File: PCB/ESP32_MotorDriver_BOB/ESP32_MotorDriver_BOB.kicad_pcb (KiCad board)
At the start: 4 copper layers, 30.5 x 58.4 mm, 39 parts, among them J1 USB_C_Receptacle_USB2.0, J2 Conn_01x06, J3 Conn_01x06, J5 Conn_01x18, J6 Conn_01x07, Q1 SSM3J338R_LF, SW1 RESET, SW2 BOOT, U1 ESP32-S2-SOLO-N4, U2 D3V3XA4B10LP, U4 TB6612FNG, U5 AP63203WU

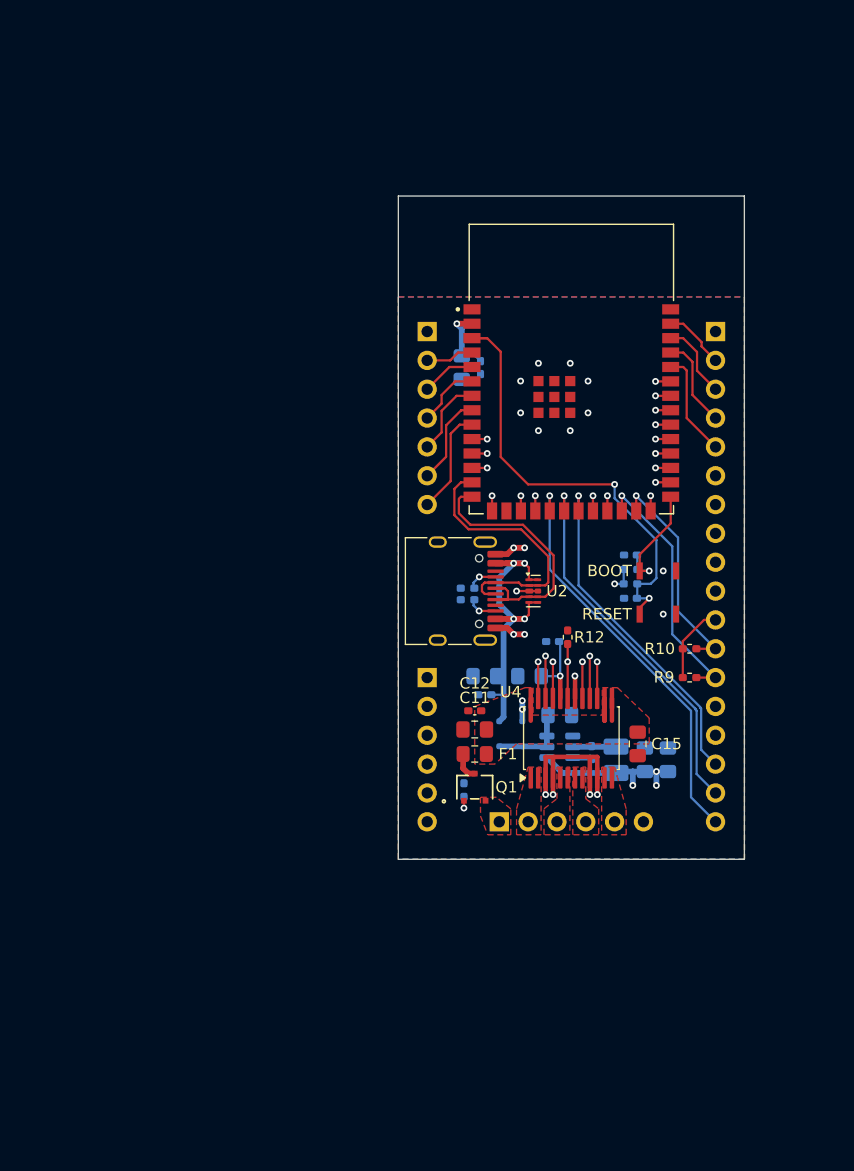
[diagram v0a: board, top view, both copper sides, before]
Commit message: actual _v01
Issue with files being copied - these should be good
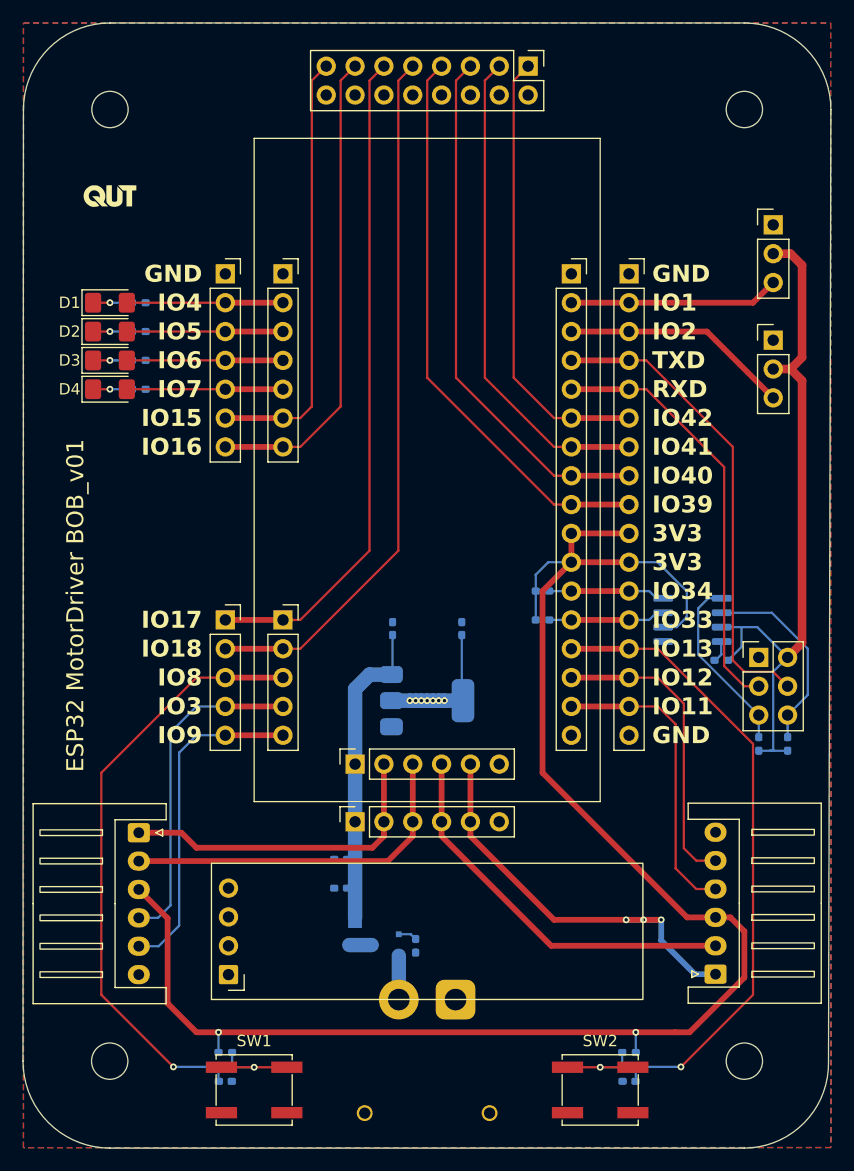
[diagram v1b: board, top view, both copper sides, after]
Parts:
- removed C1, C3, C5, C7: 10uF, Capacitor_SMD:C_0805_2012Metric_Pad1.18x1.45mm_HandSolder
- removed C10, C9: 22uF, Capacitor_SMD:C_0805_2012Metric_Pad1.18x1.45mm_HandSolder
- removed C2, C4, C6, C8: 100nF, Capacitor_SMD:C_0402_1005Metric_Pad0.74x0.62mm_HandSolder
- removed L1: 4.7uH, Inductor_SMD:L_1008_2520Metric_Pad1.43x2.20mm_HandSolder
- removed U5: AP63203WU, Package_TO_SOT_SMD:TSOT-23-6
- added C16: 100nF, Capacitor_SMD:C_0402_1005Metric_Pad0.74x0.62mm_HandSolder, B.Cu at (132.1, 113.5)
- added D3: BLUE, LED_SMD:LED_1206_3216Metric_Pad1.42x1.75mm_HandSolder, F.Cu at (86.4, 50.0)
- added D4: YELLOW, LED_SMD:LED_1206_3216Metric_Pad1.42x1.75mm_HandSolder, F.Cu at (86.4, 52.6)
- added H1: MountingHole, MountingHole:MountingHole_3.2mm_M3, F.Cu at (86.4, 27.9)
- added H2: MountingHole, MountingHole:MountingHole_3.2mm_M3, F.Cu at (142.2, 27.9)
- added H3: MountingHole, MountingHole:MountingHole_3.2mm_M3, F.Cu at (86.3, 111.8)
- added H4: MountingHole, MountingHole:MountingHole_3.2mm_M3, F.Cu at (142.2, 111.8)
- added J10: Conn_01x07, Connector_PinSocket_2.54mm:PinSocket_1x07_P2.54mm_Vertical, F.Cu at (96.5, 42.4)
- added J11: Conn_01x05, Connector_PinSocket_2.54mm:PinSocket_1x05_P2.54mm_Vertical, F.Cu at (96.5, 72.9)
- added J12: Conn_01x06, Connector_PinSocket_2.54mm:PinSocket_1x06_P2.54mm_Vertical, F.Cu at (108.0, 90.7)
- added J13: Conn_01x17, Connector_PinSocket_2.54mm:PinSocket_1x17_P2.54mm_Vertical, F.Cu at (132.1, 42.4)
- added J14: Conn_02x03_Odd_Even, Connector_PinHeader_2.54mm:PinHeader_2x03_P2.54mm_Vertical, F.Cu at (143.5, 76.2)
- added J15: Conn_02x08_Odd_Even, Connector_PinHeader_2.54mm:PinHeader_2x08_P2.54mm_Vertical, F.Cu at (123.2, 24.1)
- added J4: Conn_01x06, Connector_PinSocket_2.54mm:PinSocket_1x06_P2.54mm_Vertical, F.Cu at (108.0, 85.6)
- added J7: XT30, Connector_AMASS:AMASS_XT30PW-M_1x02_P2.50mm_Horizontal, B.Cu at (116.8, 106.3)
- added J8: Conn_01x03, Connector_PinHeader_2.54mm:PinHeader_1x03_P2.54mm_Vertical, F.Cu at (144.8, 38.1)
- added J9: Conn_01x03, Connector_PinHeader_2.54mm:PinHeader_1x03_P2.54mm_Vertical, F.Cu at (144.8, 48.3)
- added R13: 10k, Resistor_SMD:R_0402_1005Metric_Pad0.72x0.64mm_HandSolder, B.Cu at (132.1, 111.0)
- added R14: 10k, Resistor_SMD:R_0402_1005Metric_Pad0.72x0.64mm_HandSolder, B.Cu at (132.1, 112.3)
- added R5: 100k, Resistor_SMD:R_0402_1005Metric_Pad0.72x0.64mm_HandSolder, B.Cu at (140.2, 76.5)
- added R6: 4k7, Resistor_SMD:R_0402_1005Metric_Pad0.72x0.64mm_HandSolder, B.Cu at (146.1, 83.8)
- added R7: 4k7, Resistor_SMD:R_0402_1005Metric_Pad0.72x0.64mm_HandSolder, B.Cu at (143.5, 83.8)
- added R8: 4k7, Resistor_SMD:R_0402_1005Metric_Pad0.72x0.64mm_HandSolder, B.Cu at (124.5, 70.4)
- added U3: PCA9306D, Package_SO:SO-8_3.9x4.9mm_P1.27mm, B.Cu at (137.7, 72.9)
- C11: footprint Capacitor_SMD:C_0805_2012Metric_Pad1.18x1.45mm_HandSolder -> Capacitor_SMD:C_0402_1005Metric_Pad0.74x0.62mm_HandSolder; moved to B.Cu
- C12, R12, R9: moved to B.Cu
- C13, C14: value 100nF -> 10uF
- C15: value 10uF -> 100nF; footprint Capacitor_SMD:C_0805_2012Metric_Pad1.18x1.45mm_HandSolder -> Capacitor_SMD:C_0402_1005Metric_Pad0.74x0.62mm_HandSolder; moved to B.Cu
- D1: value D_Schottky -> RED; footprint Diode_SMD:D_SOD-323F -> LED_SMD:LED_1206_3216Metric_Pad1.42x1.75mm_HandSolder; moved to F.Cu
- D2: value D_Schottky -> GREEN; footprint Diode_SMD:D_SOD-323F -> LED_SMD:LED_1206_3216Metric_Pad1.42x1.75mm_HandSolder; moved to F.Cu
- F1: footprint Fuse:Fuse_0805_2012Metric_Pad1.15x1.40mm_HandSolder -> digikey-footprints:0805; moved to B.Cu
- J1: value USB_C_Receptacle_USB2.0 -> Conn_01x07; footprint Connector_USB:USB_C_Receptacle_HRO_TYPE-C-31-M-12 -> Connector_PinSocket_2.54mm:PinSocket_1x07_P2.54mm_Vertical
- J2: value Conn_01x06 -> Conn_01x05; footprint Connector_PinHeader_2.54mm:PinHeader_1x06_P2.54mm_Vertical -> Connector_PinSocket_2.54mm:PinSocket_1x05_P2.54mm_Vertical; moved to F.Cu
- J3: value Conn_01x06 -> Conn_01x17; footprint Connector_PinHeader_2.54mm:PinHeader_1x06_P2.54mm_Vertical -> Connector_PinSocket_2.54mm:PinSocket_1x17_P2.54mm_Vertical; moved to F.Cu
- J5: value Conn_01x18 -> Conn_01x06; footprint Connector_PinHeader_2.54mm:PinHeader_1x18_P2.54mm_Vertical -> Connector_JST:JST_XH_S6B-XH-A_1x06_P2.50mm_Horizontal; moved to F.Cu
- J6: value Conn_01x07 -> Conn_01x06; footprint Connector_PinHeader_2.54mm:PinHeader_1x07_P2.54mm_Vertical -> Connector_JST:JST_XH_S6B-XH-A_1x06_P2.50mm_Horizontal; moved to F.Cu
- Q1: footprint SSM3J338R_LF:SOT-23F_TOS -> SSM3J338R:SOT-23F_TOS; moved to B.Cu
- R1, R2: value 5k1 -> 150R
- R10: value 4k7 -> 10k; moved to B.Cu
- R3, R4: value 10k -> 150R
- SW1: value RESET -> SW_Push; footprint _common:Switch SMD STO -> Button_Switch_SMD:SW_SPST_EVQP0
- SW2: value BOOT -> SW_Push; footprint _common:Switch SMD STO -> Button_Switch_SMD:SW_SPST_EVQP0
- U1: value ESP32-S2-SOLO-N4 -> LDL1117S50R; footprint ESP32_S2_SOLO_N4:XCVR_ESP32-S2-SOLO-N4 -> Package_TO_SOT_SMD:SOT-223-3_TabPin2; moved to B.Cu
- U2: value D3V3XA4B10LP -> ER_OLEDM0.91_1x-I2C; footprint Package_DFN_QFN:Diodes_UDFN-10_1x2.5mm_P0.5mm -> Display:ER_OLEDM0.91_1x-I2C
- U4: value TB6612FNG -> ESP32 MotorDriver BOB_v01; footprint Package_SO:SSOP-24_5.3x8.2mm_P0.65mm -> _silkscreen:logo_QUT
- moved J5 67.3 mm to (88.9, 91.6), turned to -90 degrees
- moved U4 62.5 mm to (86.8, 35.4), turned to 0 degrees
- moved J6 62.0 mm to (139.7, 104.1), turned to 90 degrees
- moved SW1 55.0 mm to (99.1, 114.3), turned to 180 degrees
- moved D1 51.2 mm to (86.4, 45.0), turned to 0 degrees
- moved D2 50.7 mm to (86.4, 47.5), turned to 0 degrees
- moved R12 48.4 mm to (96.5, 112.3), turned to 180 degrees
- moved R3 47.6 mm to (88.9, 50.0)
- moved C15 46.9 mm to (96.5, 113.5), turned to 0 degrees
- moved R4 46.1 mm to (88.9, 52.6)
- moved SW2 46.0 mm to (129.5, 114.3), turned to 180 degrees
- moved U2 43.2 mm to (96.8, 104.1), turned to 90 degrees
- moved R1 38.4 mm to (88.9, 45.0)
- moved J3 37.8 mm to (127.0, 42.4), turned to 0 degrees
- moved R2 37.4 mm to (88.9, 47.5)
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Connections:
- C11 pad 1: VM -> Vbatt
- C12 pad 1: VM -> Vbatt
- C13 pad 1: Net-(U5-BST) -> Vbatt
- C13 pad 2: Net-(U5-SW) -> GND
- C14 pad 1: +3V3 -> +5V
- C15 pad 1: VM -> /IO8
- D1 pad 2: VBUS -> /IO4
- D2 pad 1: Net-(D1-K) -> Net-(D2-K)
- D2 pad 2: VM -> /IO5
- F1 pad 2: VM -> Vbatt
- J2 pad 1: Vbatt -> /IO17
- J2 pad 2: /M1.1 -> /IO18
- J2 pad 3: /M1.2 -> /IO8
- J2 pad 4: /M2.2 -> /IO3
- J2 pad 5: /M2.1 -> /IO9
- J3 pad 1: /IO17 -> GND
- J3 pad 2: /IO18 -> /IO1
- J3 pad 3: /IO8 -> /IO2
- J3 pad 4: /IO3 -> /TXD
- J3 pad 5: /IO9 -> /RXD
- J3 pad 6: /IO10 -> /IO42
- J5 pad 1: GND -> /M1.1
- J5 pad 2: /IO1 -> /M1.2
- J5 pad 3: /IO2 -> +3V3
- J5 pad 4: /TXD -> /IO3
- J5 pad 5: /RXD -> /IO9
- J5 pad 6: /IO42 -> GND
- J6 pad 1: GND -> /M2.1
- J6 pad 2: /IO4 -> /M2.2
- J6 pad 3: /IO5 -> +3V3
- J6 pad 4: /IO6 -> /IO11
- J6 pad 5: /IO7 -> /IO12
- J6 pad 6: /IO15 -> GND
- Q1 pad 2: Vbatt -> Net-(J7-Pin_2)
- R1 pad 1: GND -> Net-(D1-K)
- R1 pad 2: Net-(J1-CC1) -> GND
- R10 pad 1: +3V3 -> GND
- R10 pad 2: /SDA -> Net-(Q1-Pad1)
- R11 pad 1: GND -> Net-(R11-Pad1)
- R11 pad 2: Net-(Q1-Pad1) -> +3V3
- R12 pad 1: GND -> Net-(R11-Pad1)
- R12 pad 2: /M01_STBY -> /IO8
- R2 pad 1: GND -> Net-(D2-K)
- R2 pad 2: Net-(J1-CC2) -> GND
- R3 pad 1: +3V3 -> Net-(D3-K)
- R3 pad 2: /EN -> GND
- R4 pad 1: +3V3 -> Net-(D4-K)
- R4 pad 2: /BOOT -> GND
- R9 pad 1: +3V3 -> /IO33
- R9 pad 2: /SCL -> +3V3
- SW1 pad 1: /EN -> GND
- SW1 pad 2: GND -> Net-(R11-Pad1)
- SW2 pad 1: /BOOT -> GND
- SW2 pad 2: GND -> Net-(R13-Pad1)
- U1 pad 2: +3V3 -> +5V
- U1 pad 3: /EN -> Vbatt
- U2 pad 1: VBUS -> GND
- U2 pad 2: /USB_N -> +5V
- U2 pad 3: GND -> /SCL_5V0
- U2 pad 4: /USB_P -> /SDA_5V0
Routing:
- net +5V: track 0.00 -> 153.1 mm, vias 0 -> 7
- net /SCL_5V0: track 0.00 -> 74.0 mm
- net /SDA_5V0: track 0.00 -> 69.0 mm
- net +3V3: track 118.0 -> 184.9 mm, vias 6 -> 2
- net /IO13: track 0.00 -> 55.8 mm, vias 0 -> 1
- net /EN: track 40.4 -> 0.00 mm, vias 2 -> 0
- net /M2.1: track 0.00 -> 37.1 mm, vias 0 -> 3
- net /IO18: track 25.8 -> 62.0 mm, vias 1 -> 0
- net /SCK: track 36.1 -> 0.00 mm, vias 1 -> 0
- net /IO10: track 35.0 -> 0.00 mm, vias 1 -> 0
- net /IO39: track 15.6 -> 50.4 mm, vias 1 -> 0
- net /M2.2: track 0.00 -> 34.5 mm
- net /TXD: track 8.05 -> 41.9 mm
- net /IO17: track 24.5 -> 58.4 mm, vias 1 -> 0
- net /MISO: track 33.0 -> 0.00 mm, vias 1 -> 0
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- removed copper zone on F.Cu, net /M1.1
- removed copper zone on F.Cu, net /M1.2
- removed copper zone on F.Cu, net /M2.1
- removed copper zone on F.Cu, net /M2.2
- removed copper zone on F.Cu, net VM
- removed copper zone on F.Cu, net Vbatt
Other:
- board size 30.5 x 58.4 mm -> 71.2 x 99.1 mm
- board text added: "3V3"
- board text added: "GND"
- board text added: "IO1"
- board text added: "IO11"
- board text added: "IO12"
- board text added: "IO13"
- board text added: "IO15"
- board text added: "IO16"
- board text added: "IO17"
- board text added: "IO18"
- board text added: "IO2"
- board text added: "IO3"
- board text added: "IO33"
- board text added: "IO34"
- board text added: "IO39"
- board text added: "IO4"
- board text added: "IO40"
- board text added: "IO41"
- board text added: "IO42"
- board text added: "IO5"
- board text added: "IO6"
- board text added: "IO7"
- board text added: "IO8"
- board text added: "IO9"
- board text added: "RXD"
- board text added: "TXD"
